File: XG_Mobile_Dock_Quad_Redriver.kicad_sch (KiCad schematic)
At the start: 128 parts, among them J1 5-1775443-8, J13 39301240, J14 I2C1, J2 20455-040E-76, J3 20455-040E-76, J4 469911008, J7 CEE016400140111, SW1 SW_Push, U2 DS160PR410RNQR, U6 DS160PR410RNQR, U7 TPS7A8400ARGRR, U8 TPS7A8400ARGRR

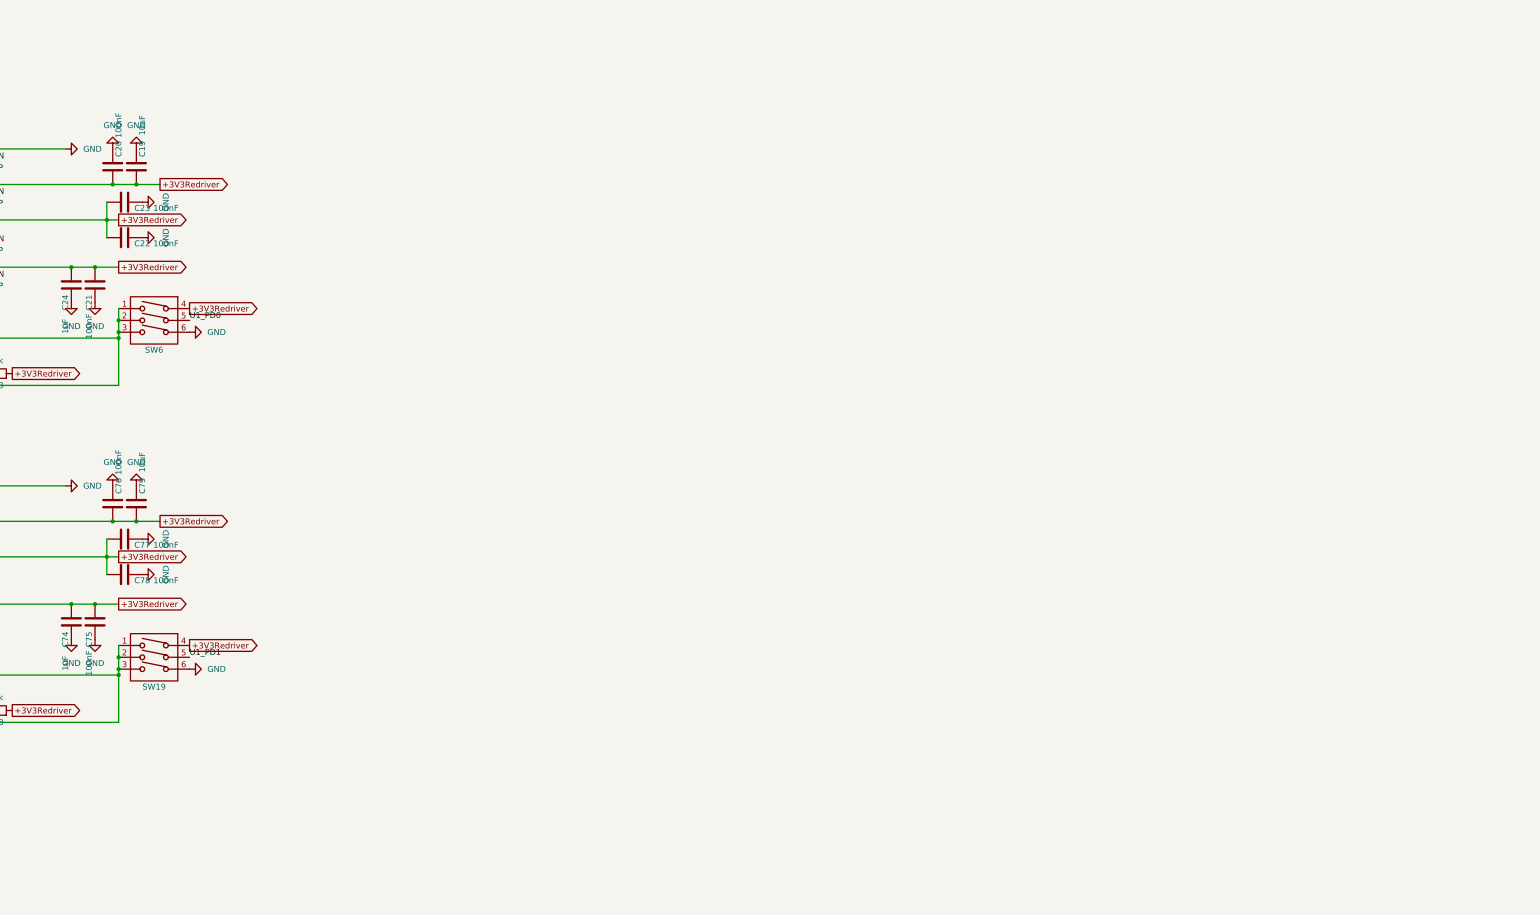
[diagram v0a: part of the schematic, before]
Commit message: quad
quad
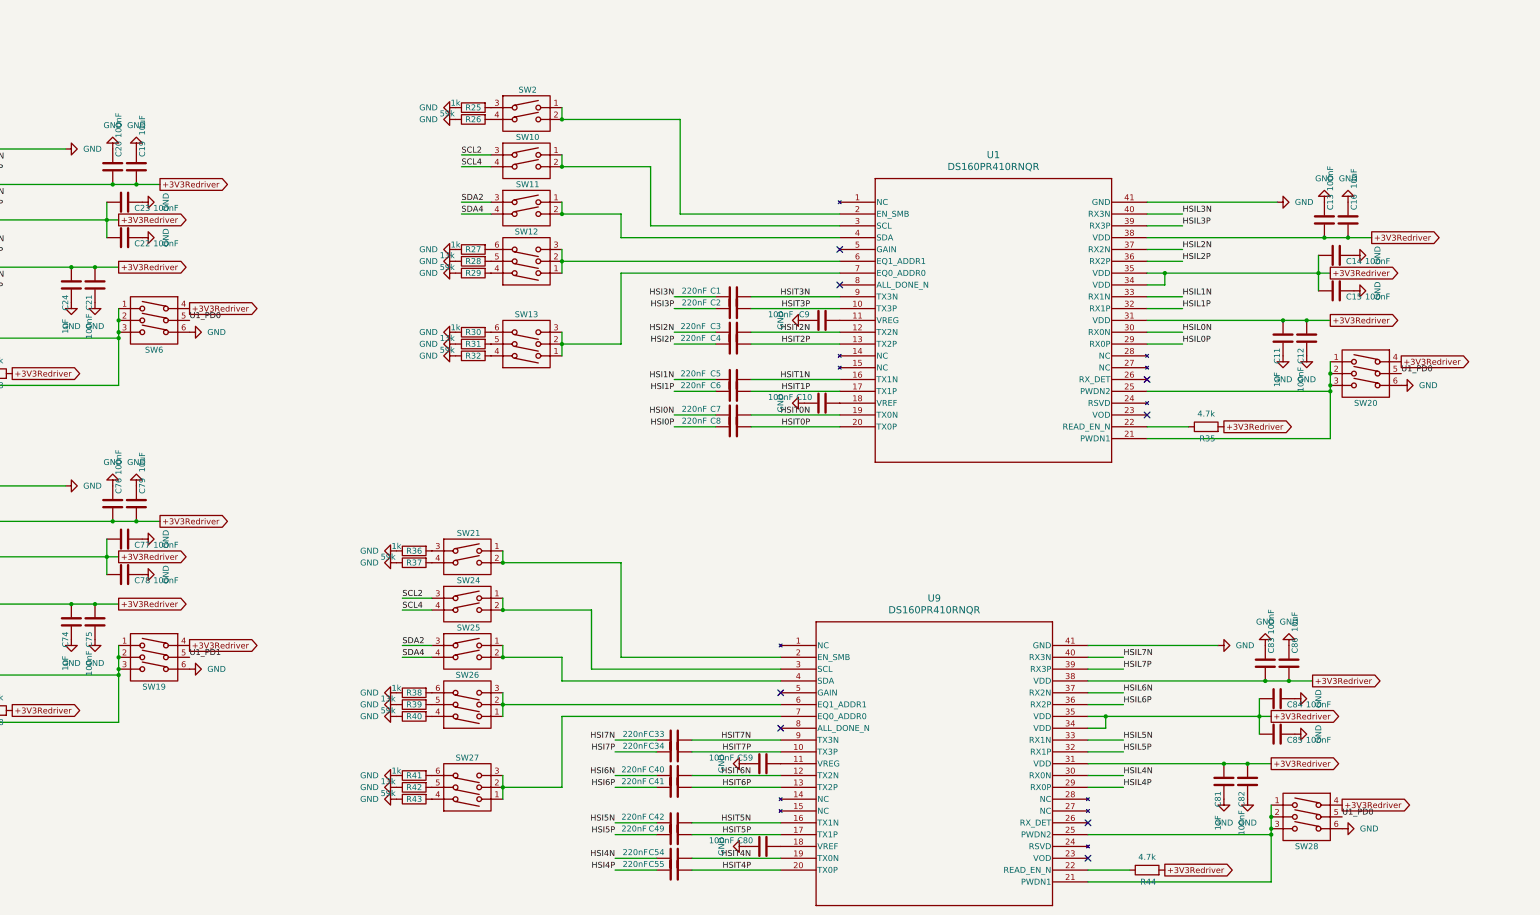
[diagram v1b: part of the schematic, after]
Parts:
- added C1, C2, C3, C33, C34, C4, C40, C41, C42, C49, C5, C54, C55, C6, C7, C8: 220nF, Capacitor_SMD:C_0201_0603Metric, symbol Device:C
- added C10, C12, C13, C14, C15, C59, C80, C82, C83, C84, C85, C9: 100nF, Capacitor_SMD:C_0201_0603Metric, symbol Device:C
- added C11, C81: 1uF, Capacitor_SMD:C_0201_0603Metric, symbol Device:C
- added C16, C86: 10uF, Capacitor_SMD:C_0603_1608Metric, symbol Device:C
- added R25, R27, R30, R36, R38, R41: 1k, Resistor_SMD:R_0603_1608Metric, symbol Device:R
- added R26, R29, R32, R37, R40, R43: 59k, Resistor_SMD:R_0603_1608Metric, symbol Device:R
- added R28, R31, R39, R42: 13k, Resistor_SMD:R_0603_1608Metric, symbol Device:R
- added R35, R44: 4.7k, Resistor_SMD:R_0402_1005Metric, symbol Device:R
- added SW10, SW11, SW2, SW21, SW24, SW25: ~, DSWB02LHGET:SW-TH_DSWB02LHGET, symbol DSWB02LHGET:DSWB02LHGET
- added SW12, SW13, SW20, SW26, SW27, SW28: ~, DSWB03LHGET:SW-TH_DSWB03LHGET, symbol DSWB03LHGET:DSWB03LHGET
- added U1, U9: DS160PR410RNQR, DS160PR410RNQR:WQFN_RNQ40_TEX, symbol DS160PR410RNQR:DS160PR410RNQR
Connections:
- net +3V3Redriver: now also C11.2, C12.2, C13.2, C14.2, C15.2, C16.2, C81.2, C82.2, C83.2, C84.2, C85.2, C86.2, R35.2, R44.2, SW20.4, SW28.4, U1.31 (VDD), U1.34 (VDD), U1.35 (VDD), U1.38 (VDD), U9.31 (VDD), U9.34 (VDD), U9.35 (VDD), U9.38 (VDD)
- net GND: now also C21.1, C10.1, C11.1, C13.1, C14.1, C15.1, C16.1, C59.1, C80.1, C81.1, C83.1, C84.1, C85.1, C86.1, C9.1, R25.1, R26.1, R27.1, R28.1, R29.1, R30.1, R31.1, R32.1, R36.1, R37.1, R38.1, R39.1, R40.1, R41.1, R42.1, R43.1, SW20.6, SW28.6, U1.41 (GND), U9.41 (GND)
- net HSI0N: now also C7.1
- net HSI0P: now also C8.1
- net HSI1N: now also C5.1
- net HSI1P: now also C6.1
- net HSI2N: now also C3.1
- net HSI2P: now also C4.1
- net HSI3N: now also C1.1
- net HSI3P: now also C2.1
- net HSI4N: now also C54.1
- net HSI4P: now also C55.1
- net HSI5N: now also C42.1
- net HSI5P: now also C49.1
- net HSI6N: now also C40.1
- net HSI6P: now also C41.1
- net HSI7N: now also C33.1
- net HSI7P: now also C34.1
- net HSIL0N: now also U1.30 (RX0N)
- net HSIL0P: now also U1.29 (RX0P)
- net HSIL1N: now also U1.33 (RX1N)
- net HSIL1P: now also U1.32 (RX1P)
- net HSIL2N: now also U1.37 (RX2N)
- net HSIL2P: now also U1.36 (RX2P)
- net HSIL3N: now also U1.40 (RX3N)
- net HSIL3P: now also U1.39 (RX3P)
- net HSIL4N: now also U9.30 (RX0N)
- net HSIL4P: now also U9.29 (RX0P)
- net HSIL5N: now also U9.33 (RX1N)
- net HSIL5P: now also U9.32 (RX1P)
- net HSIL6N: now also U9.37 (RX2N)
- net HSIL6P: now also U9.36 (RX2P)
- net HSIL7N: now also U9.40 (RX3N)
- net HSIL7P: now also U9.39 (RX3P)
- net SCL2: now also SW10.3, SW24.3
- net SCL4: now also SW10.4, SW24.4
- net SDA2: now also SW11.3, SW25.3
- net SDA4: now also SW11.4, SW25.4
- net U1_PD0: now also SW20.5, SW28.5
- new net: R35.1, U1.22 (READ_EN_N)
- new net: SW28.1, SW28.2, SW28.3, U9.21 (PWDN1), U9.25 (PWDN2)
- new net: SW10.1, SW10.2, U1.3 (SCL)
- new net: R42.2, SW27.5
- new net: SW2.1, SW2.2, U1.2 (EN_SMB)
- new net: R25.2, SW2.3
- new net: R26.2, SW2.4
- new net: R43.2, SW27.4
- new net: R30.2, SW13.6
- new net: R36.2, SW21.3
- new net: SW11.1, SW11.2, U1.4 (SDA)
- new net: C59.2, U9.11 (VREG)
- new net: SW26.1, SW26.2, SW26.3, U9.6 (EQ1_ADDR1)
- new net: R40.2, SW26.4
- new net: R39.2, SW26.5
- new net: R38.2, SW26.6
- new net: SW12.1, SW12.2, SW12.3, U1.6 (EQ1_ADDR1)
- new net: R29.2, SW12.4
- new net: R28.2, SW12.5
- new net: R27.2, SW12.6
- new net: R37.2, SW21.4
- new net: C10.2, U1.18 (VREF)
- new net: SW20.1, SW20.2, SW20.3, U1.21 (PWDN1), U1.25 (PWDN2)
- new net: C9.2, U1.11 (VREG)
- new net: SW24.1, SW24.2, U9.3 (SCL)
- new net: SW13.1, SW13.2, SW13.3, U1.7 (EQ0_ADDR0)
- new net: R32.2, SW13.4
- new net: R31.2, SW13.5
- new net: SW25.1, SW25.2, U9.4 (SDA)
- new net: R41.2, SW27.6
- new net: SW27.1, SW27.2, SW27.3, U9.7 (EQ0_ADDR0)
- new net: SW21.1, SW21.2, U9.2 (EN_SMB)
- new net: C80.2, U9.18 (VREF)
- new net: R44.1, U9.22 (READ_EN_N)
- new net HSIT0N: C7.2, U1.19 (TX0N)
- new net HSIT0P: C8.2, U1.20 (TX0P)
- new net HSIT1N: C5.2, U1.16 (TX1N)
- new net HSIT1P: C6.2, U1.17 (TX1P)
- new net HSIT2N: C3.2, U1.12 (TX2N)
- new net HSIT2P: C4.2, U1.13 (TX2P)
- new net HSIT3N: C1.2, U1.9 (TX3N)
- new net HSIT3P: C2.2, U1.10 (TX3P)
- new net HSIT4N: C54.2, U9.19 (TX0N)
- new net HSIT4P: C55.2, U9.20 (TX0P)
- new net HSIT5N: C42.2, U9.16 (TX1N)
- new net HSIT5P: C49.2, U9.17 (TX1P)
- new net HSIT6N: C40.2, U9.12 (TX2N)
- new net HSIT6P: C41.2, U9.13 (TX2P)
- new net HSIT7N: C33.2, U9.9 (TX3N)
- new net HSIT7P: C34.2, U9.10 (TX3P)
- no-connect marks 15 -> 23

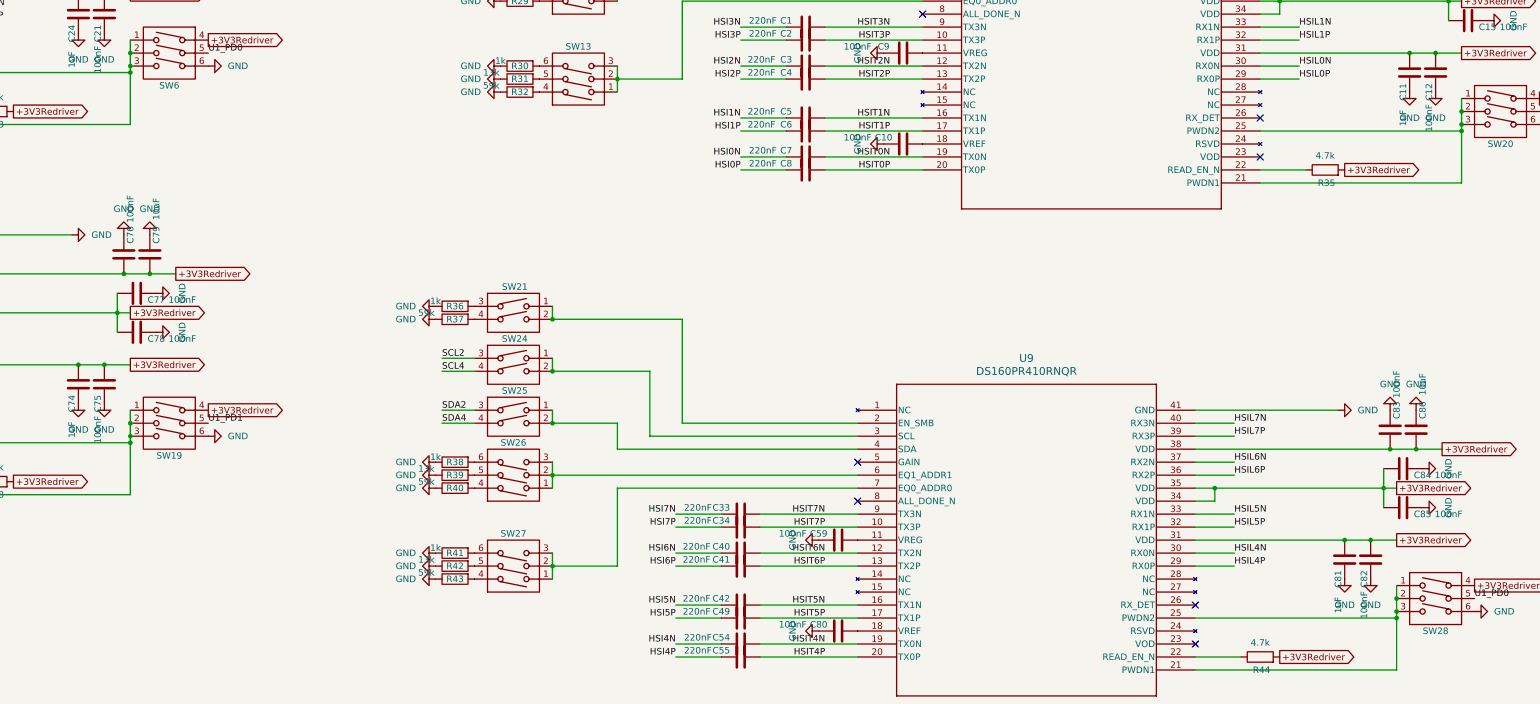
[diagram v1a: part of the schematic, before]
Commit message: quad
quad
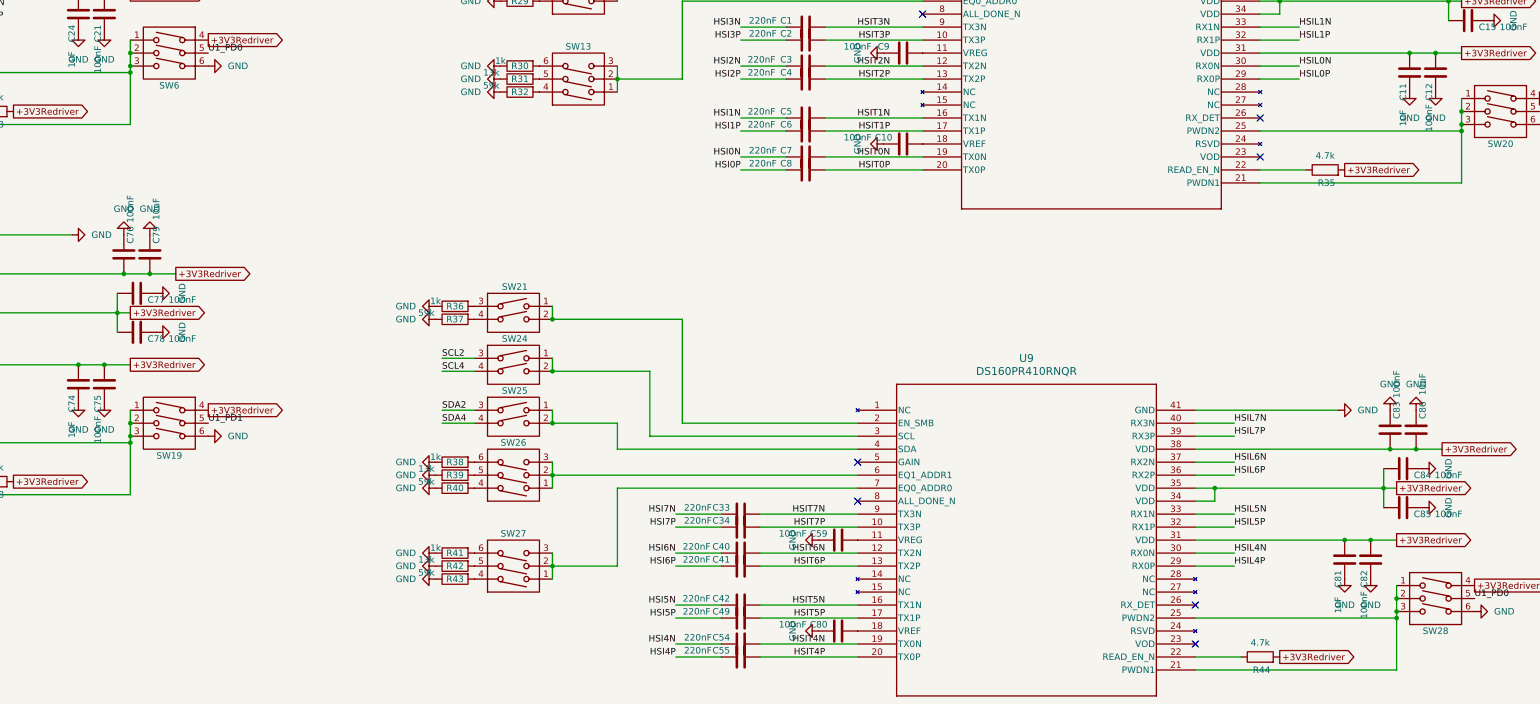
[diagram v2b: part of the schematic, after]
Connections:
- net GND: now also C12.1, C75.1, C82.1
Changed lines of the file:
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@@
 	(symbol
 		(lib_id "power:GND")
-		(at 228.6056 431.8 0)
+		(at 228.6 431.8 0)
 		(unit 1)
 		(exclude_from_sim no)
@@
 		(fields_autoplaced yes)
 		(property "Reference" "#PWR098"
-			(at 228.6056 438.15 0)
+			(at 228.6 438.15 0)
 			(effects
 				(font
@@
 		)
 		(property "Value" "GND"
-			(at 228.6056 436.88 0)
+			(at 228.6 436.88 0)
 			(effects
 				(font
@@
 		)
 		(property "Footprint" ""
-			(at 228.6056 431.8 0)
+			(at 228.6 431.8 0)
 			(effects
 				(font
@@
 		)
 		(property "Datasheet" ""
-			(at 228.6056 431.8 0)
+			(at 228.6 431.8 0)
 			(effects
 				(font
@@
 		)
 		(property "Description" "Power symbol creates a global label with name \"GND\" , ground"
-			(at 228.6056 431.8 0)
+			(at 228.6 431.8 0)
 			(effects
 				(font
@@
 	(symbol
 		(lib_id "power:GND")
-		(at 476.2556 466.09 0)
+		(at 476.25 466.09 0)
 		(unit 1)
 		(exclude_from_sim no)
@@
 		(fields_autoplaced yes)
 		(property "Reference" "#PWR093"
-			(at 476.2556 472.44 0)
+			(at 476.25 472.44 0)
 			(effects
 				(font
@@
 		)
 		(property "Value" "GND"
-			(at 476.2556 471.17 0)
+			(at 476.25 471.17 0)
 			(effects
 				(font
@@
 		)
 		(property "Footprint" ""
-			(at 476.2556 466.09 0)
+			(at 476.25 466.09 0)
 			(effects
 				(font
@@
 		)
 		(property "Datasheet" ""
-			(at 476.2556 466.09 0)
+			(at 476.25 466.09 0)
 			(effects
 				(font
@@
 		)
 		(property "Description" "Power symbol creates a global label with name \"GND\" , ground"
-			(at 476.2556 466.09 0)
+			(at 476.25 466.09 0)
 			(effects
 				(font
@@
 	(symbol
 		(lib_id "power:GND")
-		(at 488.9556 370.84 0)
+		(at 488.95 370.84 0)
 		(unit 1)
 		(exclude_from_sim no)
@@
 		(fields_autoplaced yes)
 		(property "Reference" "#PWR047"
-			(at 488.9556 377.19 0)
+			(at 488.95 377.19 0)
 			(effects
 				(font
@@
 		)
 		(property "Value" "GND"
-			(at 488.9556 375.92 0)
+			(at 488.95 375.92 0)
 			(effects
 				(font
@@
 		)
 		(property "Footprint" ""
-			(at 488.9556 370.84 0)
+			(at 488.95 370.84 0)
 			(effects
 				(font
@@
 		)
 		(property "Datasheet" ""
-			(at 488.9556 370.84 0)
+			(at 488.95 370.84 0)
 			(effects
 				(font
@@
 		)
 		(property "Description" "Power symbol creates a global label with name \"GND\" , ground"
-			(at 488.9556 370.84 0)
+			(at 488.95 370.84 0)
 			(effects
 				(font

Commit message: quadf
quadf
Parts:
- removed SW15, SW16, SW24, SW25: ~, DSWB02LHGET:SW-TH_DSWB02LHGET, symbol DSWB02LHGET:DSWB02LHGET
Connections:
- net at SW10.1, SW10.2, U1.3 (SCL): now also U9.3 (SCL)
- net at SW7.1, SW7.2, U6.3 (SCL): now also U2.3 (SCL)
- net at SW9.1, SW9.2, U6.4 (SDA): now also U2.4 (SDA)
- net at SW11.1, SW11.2, U1.4 (SDA): now also U9.4 (SDA)
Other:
- moved on the sheet: C1, C10, C11, C12, C13, C14, C15, C16, C2, C3, C33, C34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
